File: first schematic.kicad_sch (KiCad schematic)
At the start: 3 parts

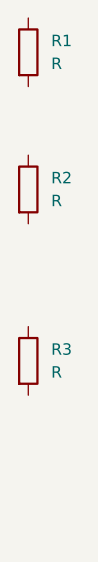
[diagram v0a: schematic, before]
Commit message: Autosave
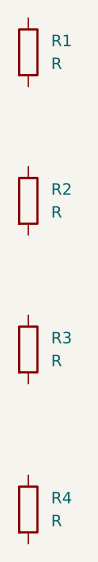
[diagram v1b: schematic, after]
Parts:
- added R4: R, symbol Device:R
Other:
- moved on the sheet: R2, R3
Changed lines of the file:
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@@
 	(symbol
 		(lib_id "Device:R")
-		(at 158.75 87.63 0)
+		(at 158.75 88.9 0)
 		(unit 1)
 		(body_style 1)
@@
 		(fields_autoplaced yes)
 		(property "Reference" "R2"
-			(at 161.29 86.3599 0)
+			(at 161.29 87.6299 0)
 			(show_name no)
 			(do_not_autoplace no)
@@
 		)
 		(property "Value" "R"
-			(at 161.29 88.8999 0)
+			(at 161.29 90.1699 0)
 			(show_name no)
 			(do_not_autoplace no)
@@
 		)
 		(property "Footprint" ""
-			(at 156.972 87.63 90)
+			(at 156.972 88.9 90)
 			(hide yes)
 			(show_name no)
@@
 		)
 		(property "Datasheet" ""
-			(at 158.75 87.63 0)
+			(at 158.75 88.9 0)
 			(hide yes)
 			(show_name no)
@@
 		)
 		(property "Description" "Resistor"
-			(at 158.75 87.63 0)
+			(at 158.75 88.9 0)
 			(hide yes)
 			(show_name no)
@@
 	(symbol
 		(lib_id "Device:R")
-		(at 158.75 106.68 0)
+		(at 158.75 105.41 0)
 		(unit 1)
 		(body_style 1)
@@
 		(fields_autoplaced yes)
 		(property "Reference" "R3"
-			(at 161.29 105.4099 0)
+			(at 161.29 104.1399 0)
 			(show_name no)
 			(do_not_autoplace no)
@@
 		)
 		(property "Value" "R"
-			(at 161.29 107.9499 0)
+			(at 161.29 106.6799 0)
 			(show_name no)
 			(do_not_autoplace no)
@@
 		)
 		(property "Footprint" ""
-			(at 156.972 106.68 90)
+			(at 156.972 105.41 90)
 			(hide yes)
 			(show_name no)
@@
 		)
 		(property "Datasheet" ""
-			(at 158.75 106.68 0)
+			(at 158.75 105.41 0)
 			(hide yes)
 			(show_name no)
@@
 		)
 		(property "Description" "Resistor"
-			(at 158.75 106.68 0)
+			(at 158.75 105.41 0)
 			(hide yes)
 			(show_name no)
@@
 					(unit 1)
 				)
+			)
+		)
+	)
+	(symbol
+		(lib_id "Device:R")
+		(at 158.75 123.19 0)
+		(unit 1)
+		(body_style 1)
+		(exclude_from_sim no)
+		(in_bom yes)
+		(on_board yes)
+		(in_pos_files yes)
+		(dnp no)
+		(fields_autoplaced yes)
+		(property "Reference" "R4"
+			(at 161.29 121.9199 0)
+			(show_name no)
+			(do_not_autoplace no)
+			(effects
+				(font
+					(size 1.27 1.27)
+				)
+				(justify left)
+			)
+		)
+		(property "Value" "R"
+			(at 161.29 124.4599 0)
+			(show_name no)
+			(do_not_autoplace no)
+			(effects
+				(font
+					(size 1.27 1.27)
+				)
+				(justify left)
+			)
+		)
+		(property "Footprint" ""
+			(at 156.972 123.19 90)
+			(hide yes)
+			(show_name no)
+			(do_not_autoplace no)
+			(effects
+				(font
+					(size 1.27 1.27)
+				)
+			)
+		)
+		(property "Datasheet" ""
+			(at 158.75 123.19 0)
+			(hide yes)
+			(show_name no)
+			(do_not_autoplace no)
+			(effects
+				(font
+					(size 1.27 1.27)
+				)
+			)
+		)
+		(property "Description" "Resistor"
+			(at 158.75 123.19 0)
+			(hide yes)
+			(show_name no)
+			(do_not_autoplace no)
+			(effects
+				(font
+					(size 1.27 1.27)
+				)
+			)
+		)
+		(pin "1"
+		)
+		(pin "2"
+		)
+		(instances
+			(project "first schematic"
+				(path "/584d0eb4-b791-43e1-a37b-188846e3a37f"
+					(reference "R4")
+					(unit 1)
+				)
